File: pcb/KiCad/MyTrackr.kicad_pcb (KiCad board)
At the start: 2 copper layers, 50 x 50 mm, 38 parts, among them CN1 GPS_ANTENNA, CON1 MICRO_SD, J1 10A45B_Module, J2 CONN_ICSP, J3 CONN_01X05, J4 CONN_BAT, P1 CONN_OLED, Q1 Q_PMOS_GSD, SW1 BTN_RESET, SW2 BTN_SEL, SW3 BTN_NEXT, SW4 BTN_PREV, SW5 BTN_BACK, U1 ATMEGA48_88_168_328P-32SMD, U2 GPS-NEO-6M, U3 24AA32

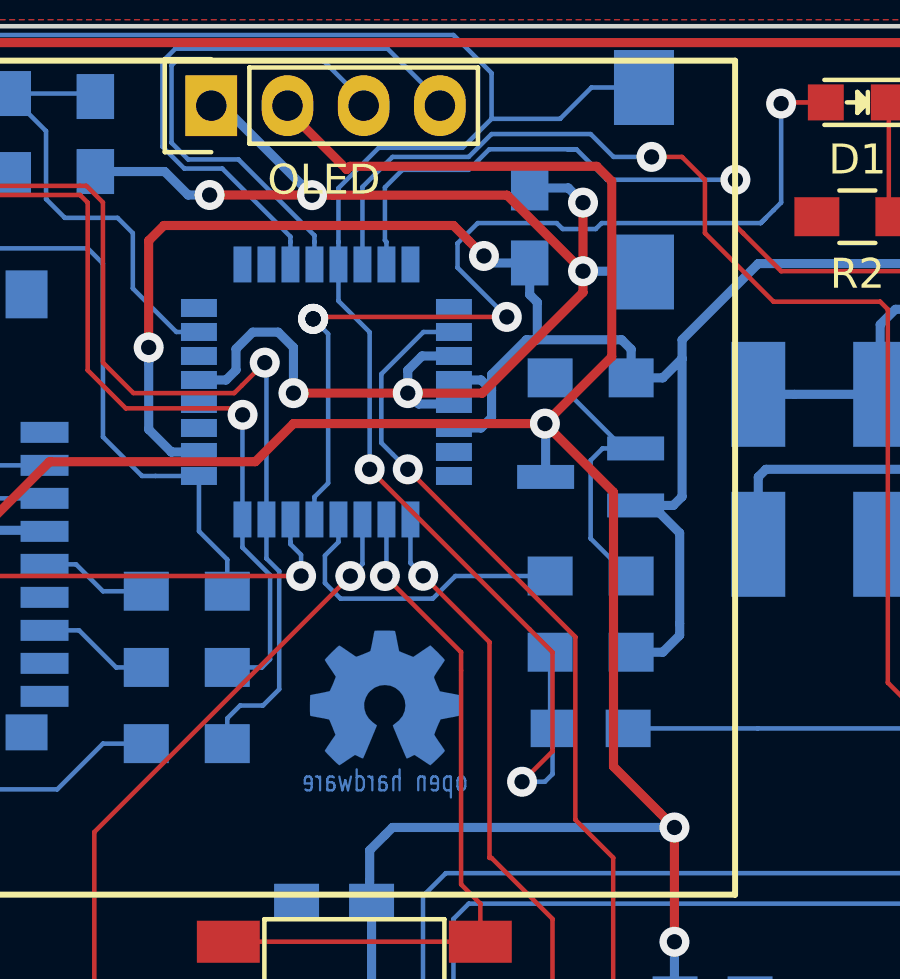
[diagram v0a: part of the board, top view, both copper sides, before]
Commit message: Expand zones
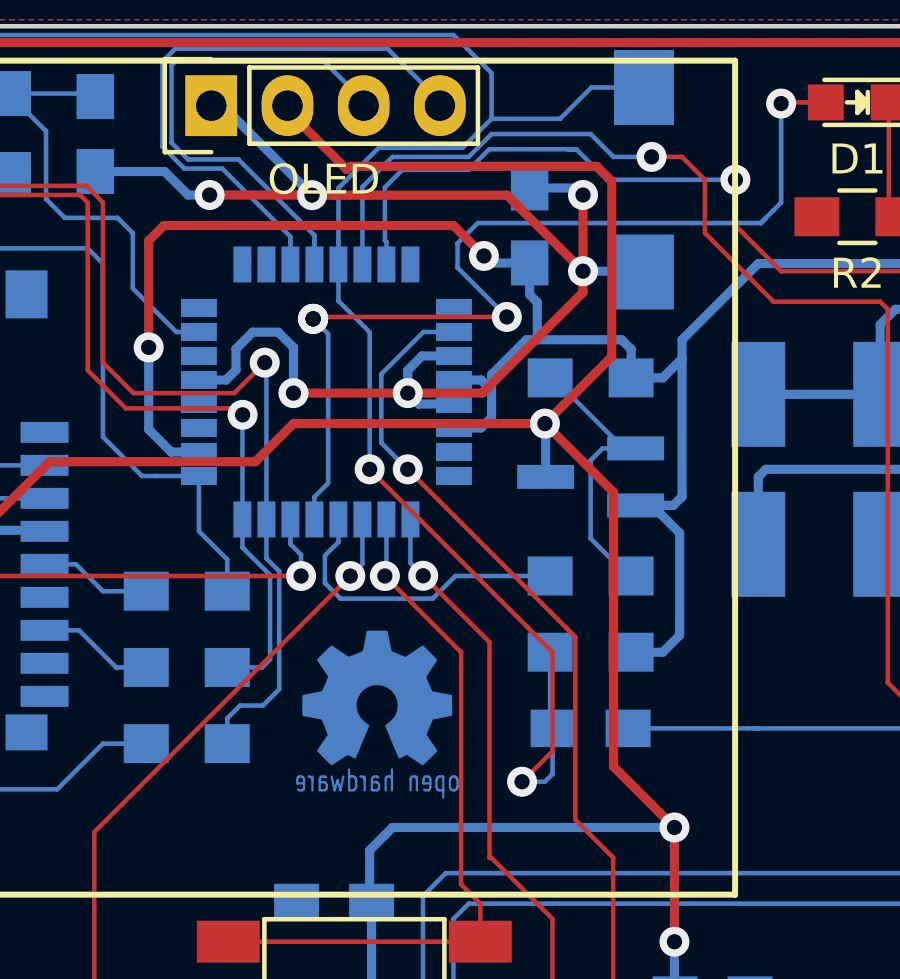
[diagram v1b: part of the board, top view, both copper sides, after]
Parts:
- moved G*** 0.25 mm to (116.3, 72.4)
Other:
- rule pad_to_mask_clearance: 0.2 -> 0
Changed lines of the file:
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@@
     (thickness 1.6)
     (drawings 39)
-    (tracks 589)
+    (tracks 586)
     (zones 0)
     (modules 38)
@@
     (last_trace_width 0.1524)
     (trace_clearance 0.1524)
-    (zone_clearance 0.2)
+    (zone_clearance 0.1524)
     (zone_45_only no)
     (trace_min 0.1524)
@@
     (mod_text_size 1 1)
     (mod_text_width 0.15)
-    (pad_size 2.032 1.7272)
-    (pad_drill 1.016)
-    (pad_to_mask_clearance 0.2)
+    (pad_size 2 0.8)
+    (pad_drill 0)
+    (pad_to_mask_clearance 0)
     (aux_axis_origin 0 0)
     (visible_elements FFFFFF7F)
@@
   (module MOUDLE-GPS-NEO-6M_24P-16X12.2MM_:GPS24P-SMD-1.1-16X12.2MM (layer B.Cu)
     (at 114.892 89.37 180)
-    (solder_mask_margin 0.1)
     (attr smd)
     (fp_text reference U2 (at -6.266 9.614 180) (layer B.SilkS)
       (effects (font (size 1 1) (thickness 0.15)) (justify mirror))
     )
-    (fp_text value GPS-NEO-6M (at 3.81 10.16 180) (layer B.SilkS) hide
+    (fp_text value GPS-NEO-6M (at 0 -1.27 180) (layer B.SilkS) hide
       (effects (font (size 1 1) (thickness 0.05)) (justify mirror))
     )
@@
     (fp_circle (center -6.985 8.255) (end -6.731 8.255) (layer B.SilkS) (width 0.508))
     (pad 1 smd rect (at -5.904 6.888) (size 2 0.8) (layers B.Cu B.Mask)
-      (solder_mask_margin 0.2))
+      (clearance 0.2))
     (pad 2 smd rect (at -5.904 5.788) (size 2 0.8) (layers B.Cu B.Mask)
-      (solder_mask_margin 0.2))
+      (clearance 0.2))
     (pad 3 smd rect (at -5.904 4.688) (size 2 0.8) (layers B.Cu B.Mask)
-      (solder_mask_margin 0.2))
+      (clearance 0.2))
     (pad 4 smd rect (at -5.904 3.588) (size 2 0.8) (layers B.Cu B.Mask)
-      (solder_mask_margin 0.2))
+      (clearance 0.2))
     (pad 5 smd rect (at -5.904 2.488) (size 2 0.8) (layers B.Cu B.Mask)
-      (solder_mask_margin 0.2))
+      (clearance 0.2))
     (pad 6 smd rect (at -5.904 1.388) (size 2 0.8) (layers B.Cu B.Mask)
-      (solder_mask_margin 0.2))
+      (clearance 0.2))
     (pad 7 smd rect (at -5.904 0.288) (size 2 0.8) (layers B.Cu B.Mask)
-      (net 2 GND) (solder_mask_margin 0.2))
+      (net 2 GND) (clearance 0.2))
     (pad 8 smd rect (at -5.904 -2.712) (size 2 0.8) (layers B.Cu B.Mask)
-      (net 25 "Net-(R3-Pad2)") (solder_mask_margin 0.2))
+      (net 25 "Net-(R3-Pad2)") (clearance 0.2))
     (pad 9 smd rect (at -5.904 -3.812) (size 2 0.8) (layers B.Cu B.Mask)
-      (net 25 "Net-(R3-Pad2)") (solder_mask_margin 0.2))
+      (net 25 "Net-(R3-Pad2)") (clearance 0.2))
     (pad 10 smd rect (at -5.904 -4.912) (size 2 0.8) (layers B.Cu B.Mask)
-      (net 2 GND) (solder_mask_margin 0.2))
+      (net 2 GND) (clearance 0.2))
     (pad 11 smd rect (at -5.904 -6.012) (size 2 0.8) (layers B.Cu B.Mask)
-      (net 13 "Net-(CN1-Pad1)") (solder_mask_margin 0.2))
+      (net 13 "Net-(CN1-Pad1)") (clearance 0.2))
     (pad 12 smd rect (at -5.904 -7.112) (size 2 0.8) (layers B.Cu B.Mask)
-      (net 2 GND) (solder_mask_margin 0.2))
+      (net 2 GND) (clearance 0.2))
     (pad 13 smd rect (at 5.896 -7.112) (size 2 0.8) (layers B.Cu B.Mask)
-      (net 2 GND) (solder_mask_margin 0.2))
+      (net 2 GND) (clearance 0.2))
     (pad 14 smd rect (at 5.896 -6.012) (size 2 0.8) (layers B.Cu B.Mask)
-      (solder_mask_margin 0.2))
+      (clearance 0.2))
     (pad 15 smd rect (at 5.896 -4.912) (size 2 0.8) (layers B.Cu B.Mask)
-      (solder_mask_margin 0.2))
+      (clearance 0.2))
     (pad 16 smd rect (at 5.896 -3.812) (size 2 0.8) (layers B.Cu B.Mask)
-      (solder_mask_margin 0.2))
+      (clearance 0.2))
     (pad 17 smd rect (at 5.896 -2.712) (size 2 0.8) (layers B.Cu B.Mask)
-      (solder_mask_margin 0.2))
+      (clearance 0.2))
     (pad 18 smd rect (at 5.896 0.288) (size 2 0.8) (layers B.Cu B.Mask)
-      (net 26 "Net-(U2-Pad18)") (solder_mask_margin 0.2))
+      (net 26 "Net-(U2-Pad18)") (clearance 0.2))
     (pad 19 smd rect (at 5.896 1.388) (size 2 0.8) (layers B.Cu B.Mask)
-      (net 27 "Net-(U2-Pad19)") (solder_mask_margin 0.2))
+      (net 27 "Net-(U2-Pad19)") (clearance 0.2))
     (pad 20 smd rect (at 5.896 2.488) (size 2 0.8) (layers B.Cu B.Mask)
-      (net 23 /GPS_TX) (solder_mask_margin 0.2))
+      (net 23 /GPS_TX))
     (pad 21 smd rect (at 5.896 3.588) (size 2 0.8) (layers B.Cu B.Mask)
-      (net 24 /GPS_RX) (solder_mask_margin 0.2))
+      (net 24 /GPS_RX) (clearance 0.2))
     (pad 22 smd rect (at 5.896 4.688) (size 2 0.8) (layers B.Cu B.Mask)
-      (net 22 "Net-(BT2-Pad1)") (solder_mask_margin 0.2))
+      (net 22 "Net-(BT2-Pad1)") (clearance 0.2))
     (pad 23 smd rect (at 5.896 5.788) (size 2 0.8) (layers B.Cu B.Mask)
-      (net 33 VPP) (solder_mask_margin 0.2))
+      (net 33 VPP) (clearance 0.2))
     (pad 24 smd rect (at 5.896 6.888) (size 2 0.8) (layers B.Cu B.Mask)
-      (net 2 GND) (solder_mask_margin 0.2))
+      (net 2 GND) (clearance 0.2))
   )
   (module MyKiCadLibs-Footprints:SW_TACT_SMD (layer F.Cu)
@@
   )
   (module w_logo:Logo_copper_OSHW_6x6mm (layer B.Cu)
-    (at 116.586 72.39 180)
+    (at 116.332 72.39 180)
     (descr "Open Hardware Logo, 6x6mm")
     (fp_text reference G*** (at 0 0 180) (layer B.SilkS) hide
@@
   (segment (start 129.286 64.77) (end 129.032 65.024) (width 0.3048) (layer B.Cu) (net 1))
   (segment (start 129.032 65.024) (end 129.032 67.26936) (width 0.3048) (layer B.Cu) (net 1))
+  (segment (start 123.19 55.626) (end 123.19 58.166) (width 0.3048) (layer F.Cu) (net 2))
+  (segment (start 121.412 55.392) (end 122.956 55.392) (width 0.3048) (layer B.Cu) (net 2))
+  (segment (start 122.956 55.392) (end 123.19 55.626) (width 0.3048) (layer B.Cu) (net 2))
+  (via (at 123.19 55.626) (size 1) (drill 0.508) (layers F.Cu B.Cu) (net 2))
   (segment (start 116.078 92.964) (end 116.078 91.694) (width 0.3048) (layer B.Cu) (net 2))
   (via (at 116.078 91.694) (size 1) (drill 0.508) (layers F.Cu B.Cu) (net 2))
@@
   (segment (start 113.03 60.198) (end 113.538 60.706) (width 0.3048) (layer B.Cu) (net 2))
   (segment (start 113.538 60.706) (end 113.538 62.23) (width 0.3048) (layer B.Cu) (net 2))
-  (segment (start 123.19 55.88) (end 123.19 58.166) (width 0.3048) (layer F.Cu) (net 2))
-  (segment (start 122.702 55.392) (end 123.19 55.88) (width 0.3048) (layer B.Cu) (net 2))
-  (segment (start 121.412 55.392) (end 122.702 55.392) (width 0.3048) (layer B.Cu) (net 2))
-  (via (at 123.19 55.88) (size 1) (drill 0.508) (layers F.Cu B.Cu) (net 2))
   (segment (start 110.744 55.626) (end 114.15137 55.626) (width 0.3048) (layer F.Cu) (net 2))
   (segment (start 114.15137 55.626) (end 114.15699 55.63162) (width 0.3048) (layer F.Cu) (net 2))
@@
   (segment (start 137.5156 74.676) (end 137.668 74.676) (width 0.1524) (layer F.Cu) (net 18))
   (segment (start 122.682 54.102) (end 122.936 54.102) (width 0.1524) (layer B.Cu) (net 18))
+  (segment (start 120.65 59.69) (end 119.006998 58.046998) (width 0.1524) (layer B.Cu) (net 19))
+  (segment (start 119.006998 58.046998) (end 119.006998 57.235118) (width 0.1524) (layer B.Cu) (net 19))
+  (segment (start 119.006998 57.235118) (end 119.680117 56.561999) (width 0.1524) (layer B.Cu) (net 19))
+  (segment (start 119.680117 56.561999) (end 123.811885 56.561999) (width 0.1524) (layer B.Cu) (net 19))
+  (segment (start 123.811885 56.561999) (end 129.112001 56.561999) (width 0.1524) (layer B.Cu) (net 19))
   (segment (start 129.794 52.578) (end 129.794 55.88) (width 0.1524) (layer B.Cu) (net 19))
   (segment (start 129.794 55.88) (end 129.54 56.134) (width 0.1524) (layer B.Cu) (net 19))
@@
   (segment (start 114.238 65.6896) (end 114.694193 65.233407) (width 0.1524) (layer B.Cu) (net 19))
   (segment (start 114.694193 65.233407) (end 114.694193 60.254493) (width 0.1524) (layer B.Cu) (net 19))
-  (segment (start 122.513118 56.761002) (end 123.612882 56.761002) (width 0.1524) (layer B.Cu) (net 19))
-  (segment (start 122.314115 56.561999) (end 122.513118 56.761002) (width 0.1524) (layer B.Cu) (net 19))
-  (segment (start 120.65 59.69) (end 119.006998 58.046998) (width 0.1524) (layer B.Cu) (net 19))
-  (segment (start 123.811885 56.561999) (end 129.112001 56.561999) (width 0.1524) (layer B.Cu) (net 19))
-  (segment (start 119.680117 56.561999) (end 122.314115 56.561999) (width 0.1524) (layer B.Cu) (net 19))
-  (segment (start 119.006998 57.235118) (end 119.680117 56.561999) (width 0.1524) (layer B.Cu) (net 19))
-  (segment (start 123.612882 56.761002) (end 123.811885 56.561999) (width 0.1524) (layer B.Cu) (net 19))
-  (segment (start 119.006998 58.046998) (end 119.006998 57.235118) (width 0.1524) (layer B.Cu) (net 19))
   (via (at 120.65 59.69) (size 1) (drill 0.508) (layers F.Cu B.Cu) (net 19))
   (segment (start 129.112001 56.561999) (end 129.54 56.134) (width 0.1524) (layer B.Cu) (net 19))
@@
   (segment (start 123.8416 64.074) (end 124.944 64.074) (width 0.1524) (layer B.Cu) (net 36))
   (zone (net 2) (net_name GND) (layer F.Cu) (hatch edge 0.508)
-    (connect_pads (clearance 0.2))
-    (min_thickness 0.1)
-    (fill (arc_segments 16) (thermal_gap 0.508) (thermal_bridge_width 0.508))
+    (connect_pads (clearance 0.1524))
+    (min_thickness 0.0254)
+    (fill yes (arc_segments 16) (thermal_gap 0.1524) (thermal_bridge_width 0.254))
     (polygon
       (pts
@@
   )
   (zone (net 2) (net_name GND) (layer B.Cu) (hatch edge 0.508)
-    (connect_pads (clearance 0.2))
-    (min_thickness 0.1)
-    (fill (arc_segments 16) (thermal_gap 0.508) (thermal_bridge_width 0.508))
+    (connect_pads (clearance 0.1524))
+    (min_thickness 0.0254)
+    (fill yes (arc_segments 16) (thermal_gap 0.1524) (thermal_bridge_width 0.254))
     (polygon
       (pts
